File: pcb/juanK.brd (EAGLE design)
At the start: 138.1 x 97.8 mm, 57 parts, among them IC1 MEGA8-P, IC2 7805TV, T1 2N3904, T2 MCR106, T3 MCR106, T4 MCR106, T5 MCR106, T6 MCR106, T7 MCR106

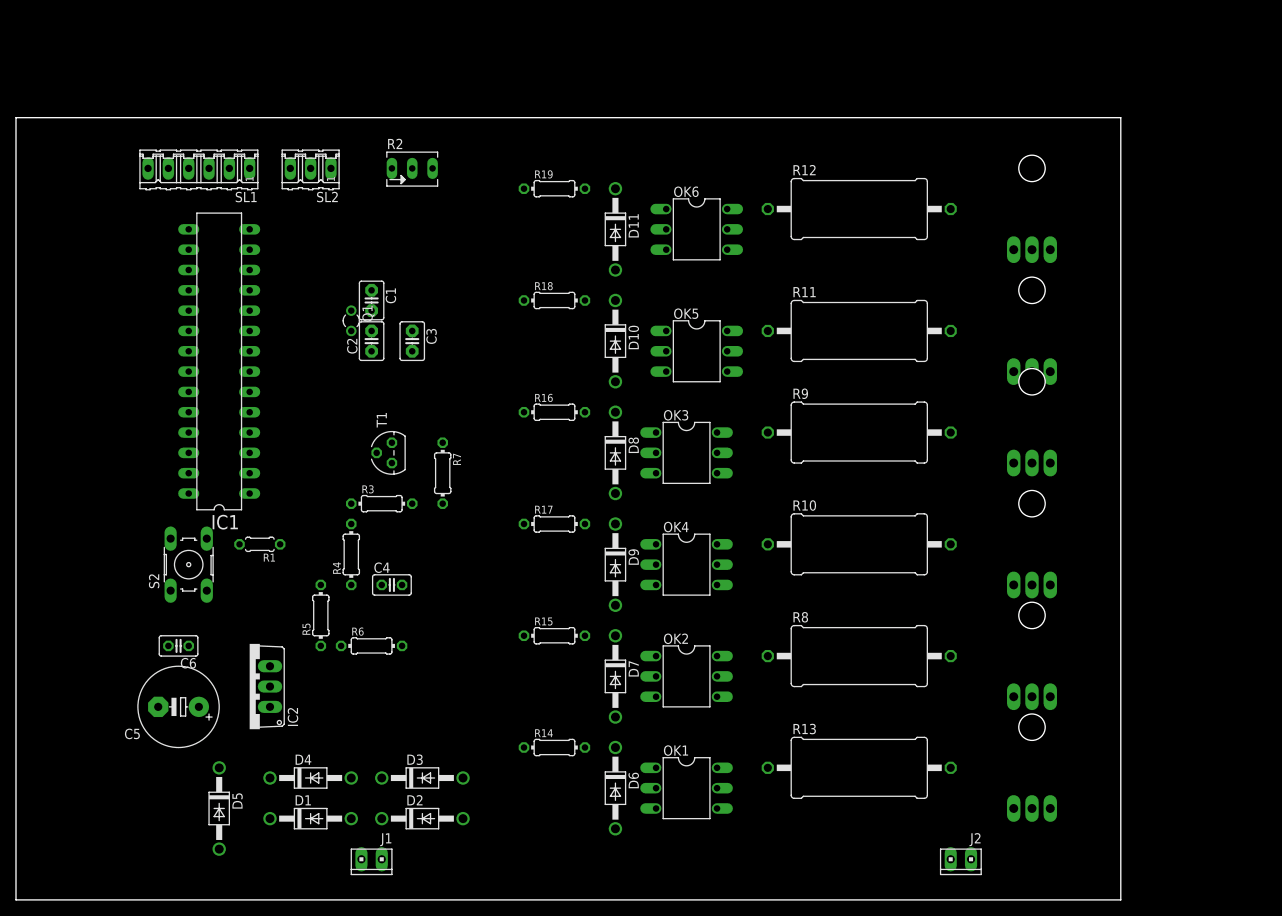
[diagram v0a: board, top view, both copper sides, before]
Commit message: Diseño de PCB terminado
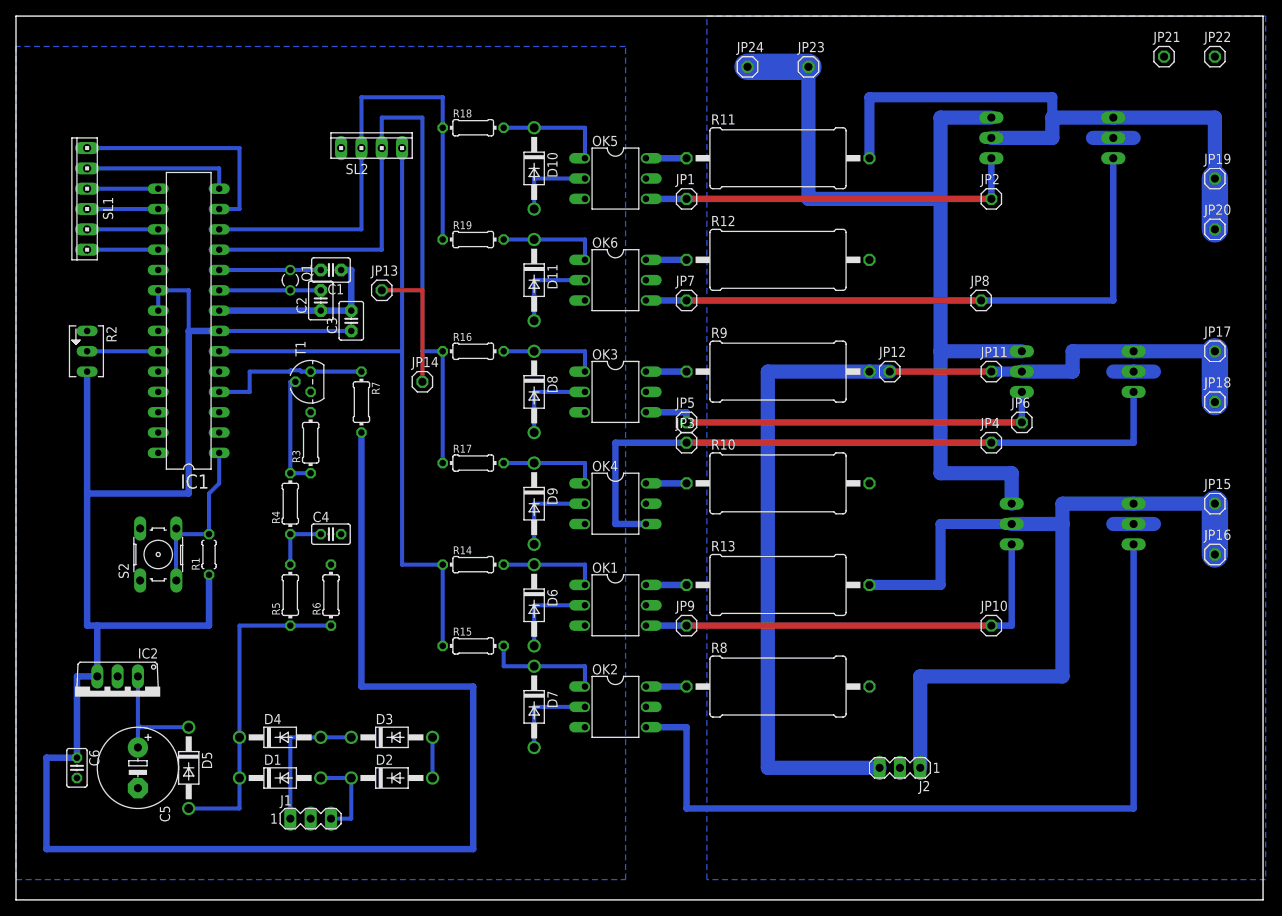
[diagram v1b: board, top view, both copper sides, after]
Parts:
- added JP1, JP10, JP11, JP12, JP13, JP14, JP15, JP16, JP17, JP18, JP19, JP2, JP20, JP21, JP22, JP23, JP24, JP3, JP4, JP5, JP6, JP7, JP8, JP9: (no value), pinhead:1X01
- J1, J2: device con-amp:10X02MTA -> con-lstb:MA03-1
- SL1: device con-amp-quick:06P -> con-amp:10X06MTA
- SL2: device con-amp-quick:03P -> con-amp:10X04MTA
- T2, T3, T4, T5, T6, T7: value MCR106 -> TIC106S; device triac:TO126L -> triac:TIC106S
- moved R2 46.6 mm to (8.89, 68.6), turned to 270 degrees
- moved T2 30.9 mm to (121.9, 47.0), turned to 270 degrees
- moved T6 25.3 mm to (119.4, 95.2), turned to 270 degrees
- moved D6 25.0 mm to (64.8, 36.8)
- moved R13 25.0 mm to (95.2, 39.4)
- moved R14 25.0 mm to (57.1, 41.9)
- moved OK1 24.5 mm to (74.9, 36.8)
- moved D10 23.9 mm to (64.8, 91.4)
- moved OK5 23.9 mm to (74.9, 90.2)
- moved T5 23.9 mm to (137.2, 66.0), turned to 270 degrees
- moved R18 23.9 mm to (57.1, 96.5)
- moved R11 23.9 mm to (95.2, 92.7)
- moved C6 19.8 mm to (7.62, 16.5), turned to 270 degrees
- moved T3 19.4 mm to (137.2, 47.0), turned to 270 degrees
- moved IC2 16.6 mm to (12.7, 25.4), turned to 180 degrees
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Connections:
- removed net N$13: T2.C, T4.C, T6.C
- new net VO: JP23.1, JP24.1, T2.C, T4.C, T6.C
- net A: now also JP15.1, JP16.1
- net B: now also J2.3, JP11.1, JP12.1, JP17.1, JP18.1; no longer J2.2
- net C: now also JP19.1, JP20.1
- net GND: now also JP13.1, JP14.1, SL2.4
- net GND1: now also JP21.1, JP22.1
- net N$11: now also J1.3; no longer J1.2
- net N$22: now also JP5.1, JP6.1
- net N$24: now also JP7.1, JP8.1
- net N$25: now also JP3.1, JP4.1
- net N$6: now also JP10.1, JP9.1
- net N$8: now also JP1.1, JP2.1
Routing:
- net 5V: track 0.00 -> 272.0 mm
- net B: track 0.00 -> 128.3 mm
- net VO: track 0.00 -> 114.3 mm
- net A: track 0.00 -> 108.0 mm
- net N$20: track 0.00 -> 104.1 mm
- net S1_S2: track 0.00 -> 90.2 mm
- net S3_S4: track 0.00 -> 87.6 mm
- net N$25: track 0.00 -> 85.1 mm
- net C: track 0.00 -> 77.5 mm
- net N$24: track 0.00 -> 76.2 mm
- net S5_S6: track 0.00 -> 62.2 mm
- net N$6: track 0.00 -> 55.9 mm
- net N$22: track 0.00 -> 52.1 mm
- net N$8: track 0.00 -> 48.3 mm
- net GND: track 0.00 -> 44.4 mm
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- added copper zone on layer 16, net GND
- added copper zone on layer 16, net GND1
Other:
- board size 138.1 x 97.8 mm -> 155.9 x 110.5 mm
